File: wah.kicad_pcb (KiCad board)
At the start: 4 copper layers, 99.1 x 54.5 mm, 38 parts, among them J1 Barrel_Jack_Switch, J2 In, J3 Out, SW1 SW_Push_3PDT, U1 TL072, U2 L78L05_TO92

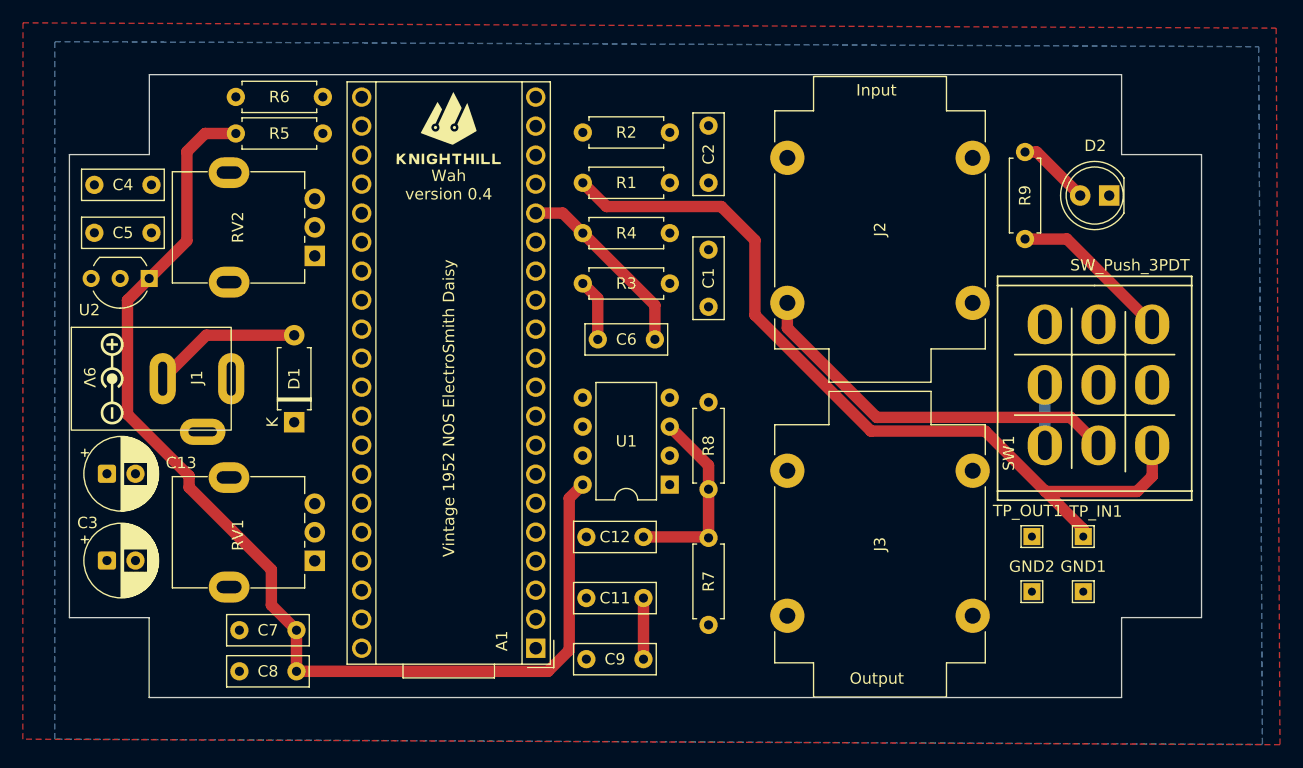
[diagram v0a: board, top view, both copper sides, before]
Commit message: polish pcb
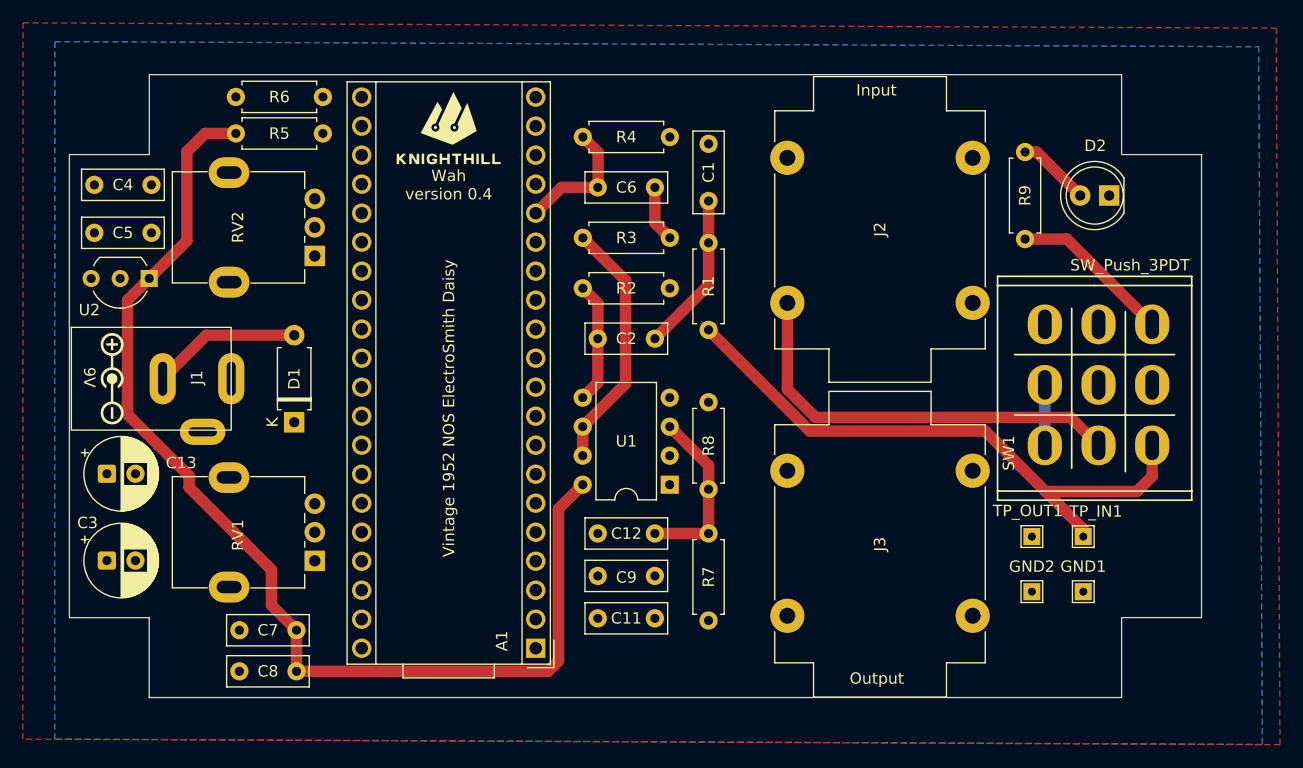
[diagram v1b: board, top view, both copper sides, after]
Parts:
- moved R1 16.9 mm to (98.4, 55.5), turned to 90 degrees
- moved R2 15.6 mm to (95.0, 51.9), turned to 180 degrees
- moved C2 14.4 mm to (93.7, 56.3), turned to 180 degrees
- moved C6 14.2 mm to (93.7, 43.1), turned to 180 degrees
- moved R3 8.60 mm to (87.4, 47.5), turned to 0 degrees
- moved R4 8.42 mm to (87.4, 38.6)
- moved C9 8.32 mm to (88.7, 77.1), turned to 0 degrees
- moved C11 4.38 mm to (88.7, 80.8), turned to 0 degrees
- moved C1 4.27 mm to (98.4, 44.2), turned to 90 degrees
- moved C12 1.05 mm to (93.7, 73.4)
- moved R7 0.39 mm to (98.4, 81.0)
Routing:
- net /FX_IN: track 73.5 -> 53.3 mm
- net Net-(U1B-+): track 30.0 -> 10.7 mm
- net Net-(C11-Pad2): track 11.7 -> 4.78 mm
- net /AUDIO_IN: track 16.8 -> 11.3 mm
- net Net-(C1-Pad1): track 9.25 -> 14.0 mm
- net Net-(U1B--): track 18.2 -> 22.2 mm
- net Net-(J2-PadT): track 33.7 -> 36.9 mm
- net /AUDIO_OUT: track 48.0 -> 45.0 mm
- net Net-(U1A-+): track 16.9 -> 15.5 mm
